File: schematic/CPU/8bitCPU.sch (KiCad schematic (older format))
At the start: 25 parts, among them U77 74LS245

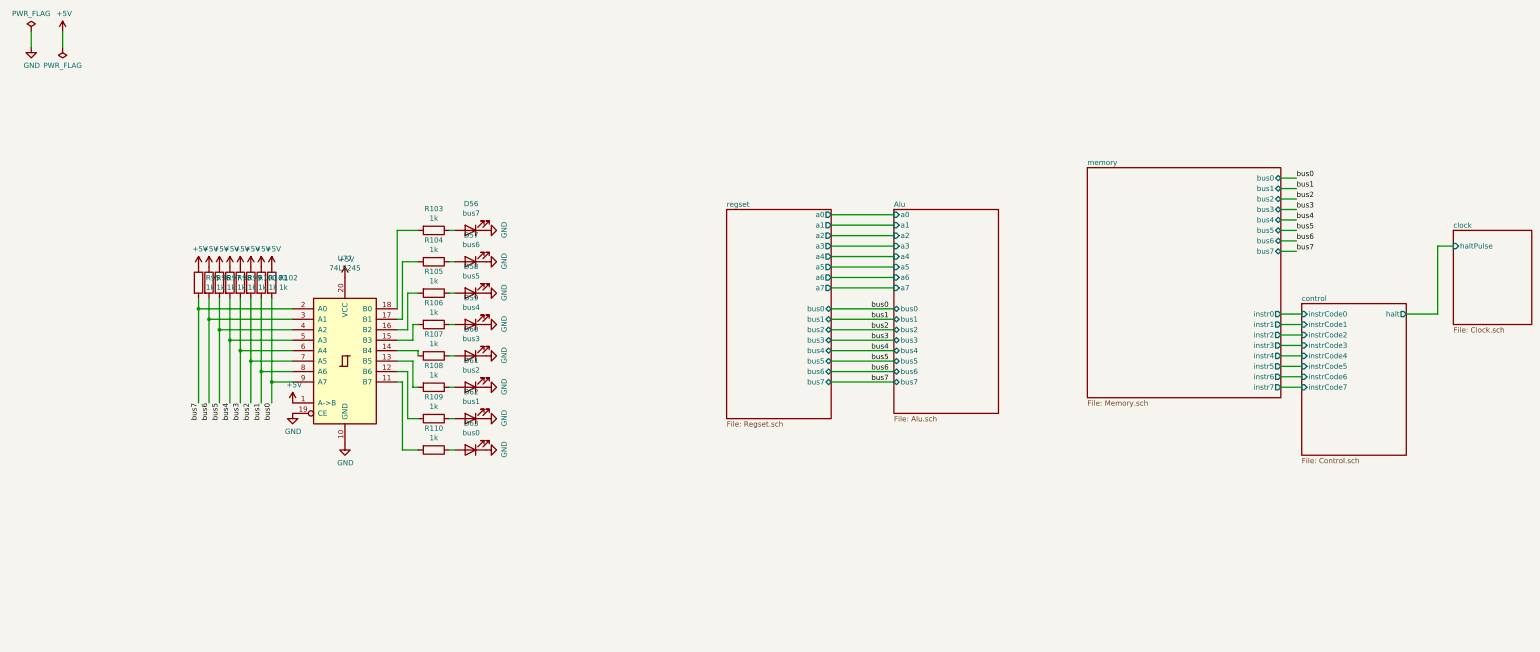
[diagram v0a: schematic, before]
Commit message: schematic with henry
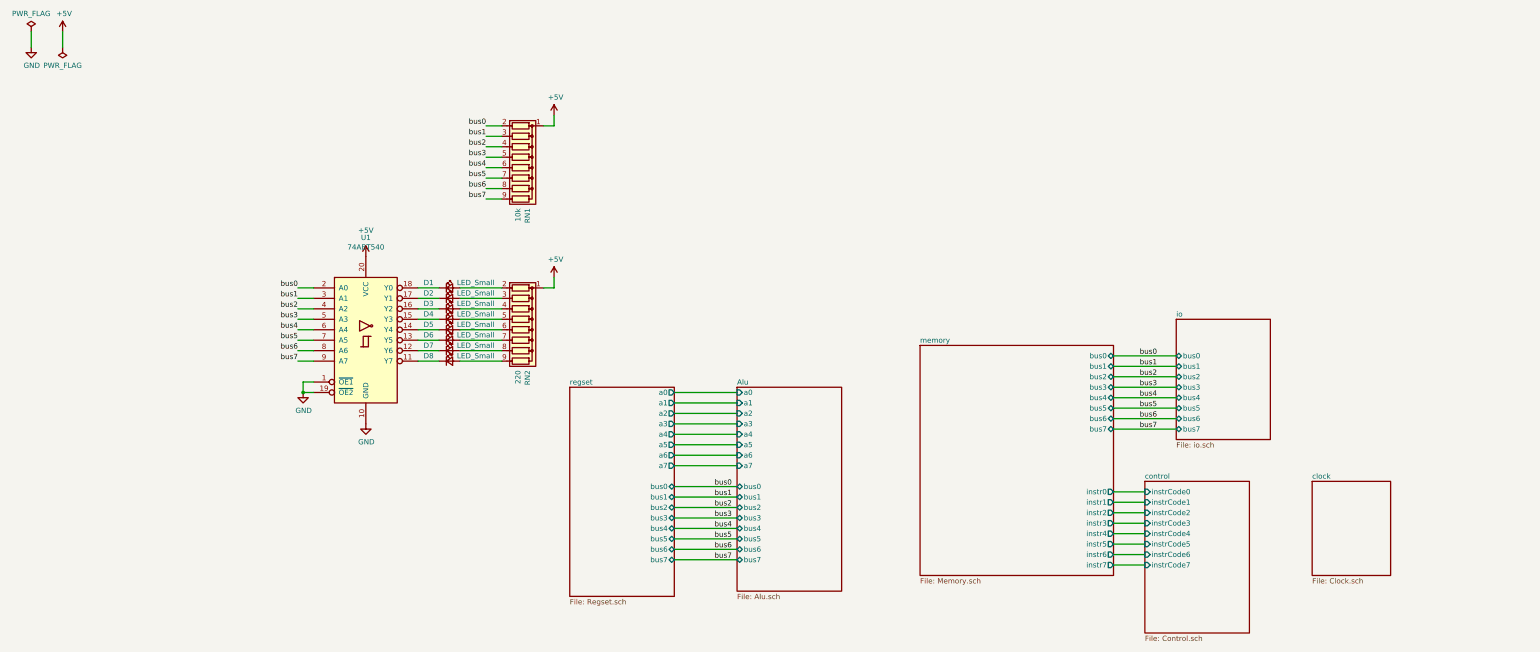
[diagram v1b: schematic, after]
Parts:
- removed D56: bus7, LED_THT:LED_D3.0mm, symbol Device:LED
- removed D57: bus6, LED_THT:LED_D3.0mm, symbol Device:LED
- removed D58: bus5, LED_THT:LED_D3.0mm, symbol Device:LED
- removed D59: bus4, LED_THT:LED_D3.0mm, symbol Device:LED
- removed D60: bus3, LED_THT:LED_D3.0mm, symbol Device:LED
- removed D61: bus2, LED_THT:LED_D3.0mm, symbol Device:LED
- removed D62: bus1, LED_THT:LED_D3.0mm, symbol Device:LED
- removed D63: bus0, LED_THT:LED_D3.0mm, symbol Device:LED
- removed R100, R101, R102, R95, R96, R97, R98, R99: 1k, symbol Device:R
- removed R103, R104, R105, R106, R107, R108, R109, R110: 1k, Resistor_THT:R_Axial_DIN0207_L6.3mm_D2.5mm_P7.62mm_Horizontal, symbol Device:R
- removed U77: 74LS245, symbol 74xx:74LS245
- added D1, D2, D3, D4, D5, D6, D7, D8: LED_Small, symbol Device:LED_Small
- added RN1: 10k, Resistor_THT:R_Array_SIP9, symbol Device:R_Network08
- added RN2: 220, Resistor_THT:R_Array_SIP9, symbol Device:R_Network08
- added U1: 74ABT540, symbol 8bitCPU-rescue:74ABT540
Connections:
- net +5V: now also RN1.1 (common), RN2.1 (common), U1.20 (VCC)
- net GND: now also U1.1 (~OE1~), U1.10 (GND), U1.19 (~OE2~)
- net bus0: now also RN1.2 (R1), U1.2 (A0)
- net bus1: now also RN1.3 (R2), U1.3 (A1)
- net bus2: now also RN1.4 (R3), U1.4 (A2)
- net bus3: now also RN1.5 (R4), U1.5 (A3)
- net bus4: now also RN1.6 (R5), U1.6 (A4)
- net bus5: now also RN1.7 (R6), U1.7 (A5)
- net bus6: now also RN1.8 (R7), U1.8 (A6)
- net bus7: now also RN1.9 (R8), U1.9 (A7)
- new net: D8.1 (K), U1.11 (Y7)
- new net: D7.1 (K), U1.12 (Y6)
- new net: D6.1 (K), U1.13 (Y5)
- new net: D5.1 (K), U1.14 (Y4)
- new net: D4.1 (K), U1.15 (Y3)
- new net: D3.1 (K), U1.16 (Y2)
- new net: D2.1 (K), U1.17 (Y1)
- new net: D1.1 (K), U1.18 (Y0)
- new net: D1.2 (A), RN2.2 (R1)
- new net: D2.2 (A), RN2.3 (R2)
- new net: D3.2 (A), RN2.4 (R3)
- new net: D4.2 (A), RN2.5 (R4)
- new net: D5.2 (A), RN2.6 (R5)
- new net: D6.2 (A), RN2.7 (R6)
- new net: D7.2 (A), RN2.8 (R7)
- new net: D8.2 (A), RN2.9 (R8)
